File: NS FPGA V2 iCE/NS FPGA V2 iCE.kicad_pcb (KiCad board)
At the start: 4 copper layers, 27 x 55.5 mm, 70 parts, among them J1 USB_C_Receptacle_USB2.0_14P, J2 Conn_01x20_Pin, J3 Conn_01x20_Pin, J4 Conn_02x03_Odd_Even, J5 Conn_02x03_Odd_Even, J6 Conn_01x07_Pin, SW1 SW_Push, U1 ICE40UP5K-SG48ITR, U2 W25Q128JVS, U3 CP2102N-Axx-xQFN24, U4 AP2112K-3.3, U5 AP2112K-1.2, U6 AP2112K-2.5, U7 AP2112K-1.8, Y1 SG-210STF

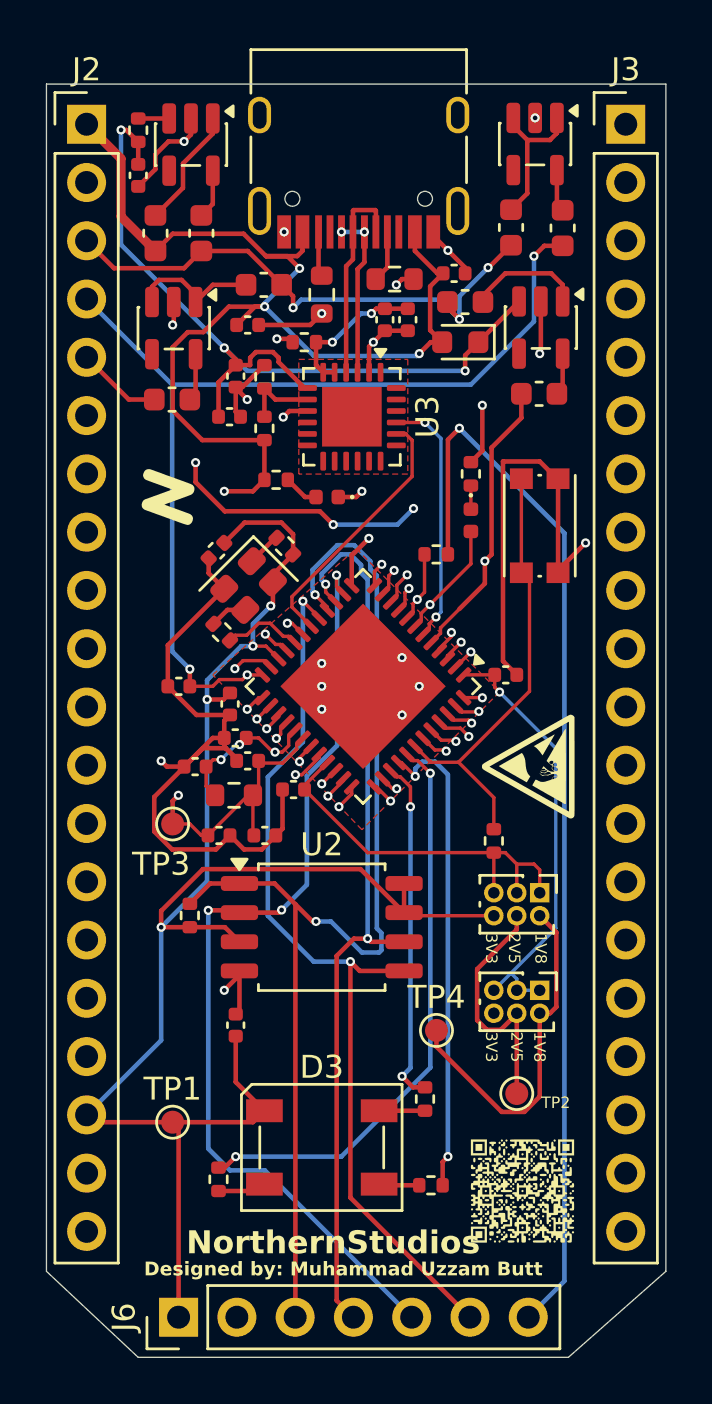
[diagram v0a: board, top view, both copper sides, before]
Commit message: done with BOM/CPL
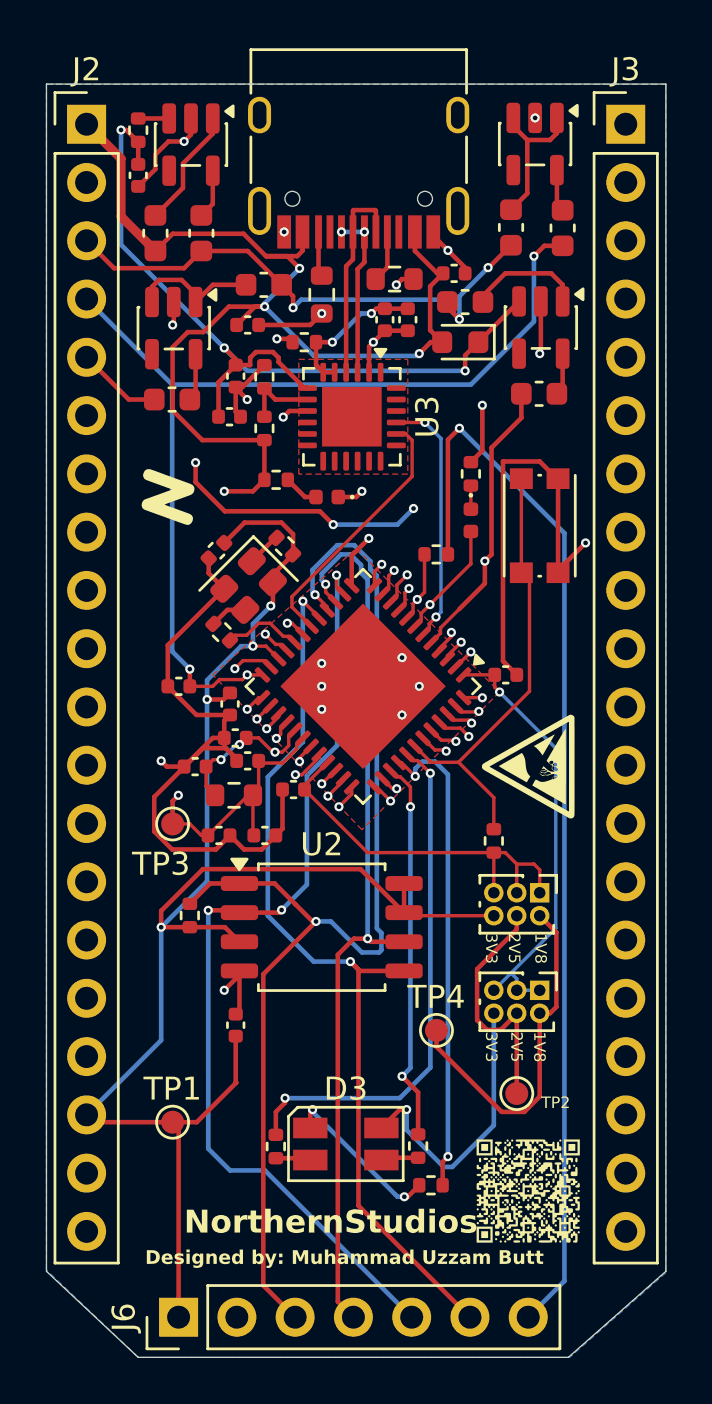
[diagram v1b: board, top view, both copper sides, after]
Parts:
- D3: footprint LED_SMD:LED_Cree-PLCC4_5x5mm_CW -> LED_SMD:LED_RGB_Wuerth-PLCC4_3.2x2.8mm_150141M173100
- moved R14 2.88 mm to (187.0, 98.3)
- moved R12 2.07 mm to (193.2, 98.3)
- moved D3 1.06 mm to (190.1, 98.2)
- moved G*** 0.25 mm to (198.0, 100.2)
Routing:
- net +3V3: track 133.3 -> 143.2 mm, vias 7 -> 8
- net Net-(D3-GK): track 1.77 -> 7.33 mm, vias 0 -> 2
- net Net-(U1A-RGB2): track 25.2 -> 22.8 mm
- net Net-(U1A-RGB0): track 15.1 -> 16.7 mm
- net /SPI_SS: track 50.4 -> 51.2 mm
- net Net-(D3-BK): track 2.12 -> 1.53 mm
- added copper zone on B.Cu, net +3V3
